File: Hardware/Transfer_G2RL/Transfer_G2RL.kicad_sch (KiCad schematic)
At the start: 20 parts, among them J1 Screw_Terminal_01x02, J5 SO-239, J6 SO-239, J7 SO-239, J8 SO-239, K2 G2RL-1-E, K3 G2RL-1-E

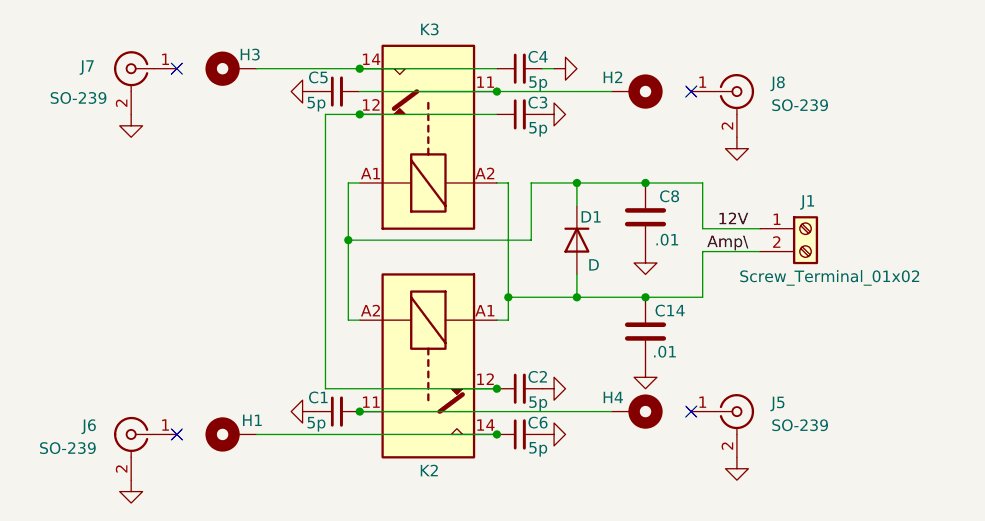
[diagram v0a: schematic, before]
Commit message: replacing through holes with surface pads for RF to coax center pin wires
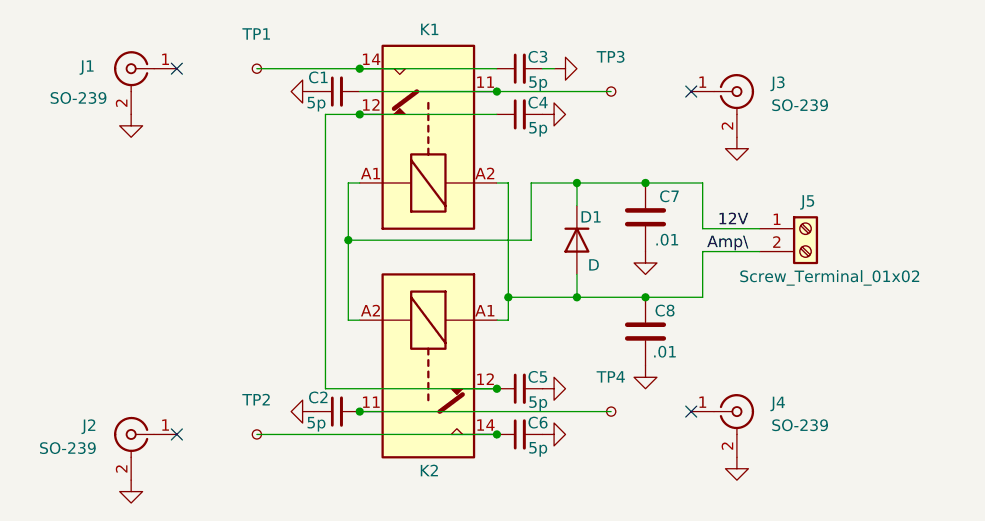
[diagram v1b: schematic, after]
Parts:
- removed H1, H2, H3, H4: MountingHole_Pad, TestPoint:TestPoint_Plated_Hole_D2.0mm, symbol Mechanical:MountingHole_Pad
- added TP1, TP2, TP3, TP4: ~, TestPoint:TestPoint_Pad_3.0x3.0mm, symbol Connector:TestPoint_Small
- renumbered C5 to C1, C1 to C2, C4 to C3, C3 to C4, C2 to C5, C8 to C7, C14 to C8, J7 to J1, J6 to J2, J8 to J3, J5 to J4, J1 to J5, K3 to K1
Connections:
- net at C1.2, K1.11: now also TP3.1
- net at C2.2, K2.11: now also TP4.1
- net at C3.1, K1.14: now also TP1.1
- net at C6.1, K2.14: now also TP2.1

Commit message: Manually merged git branch V2 into main
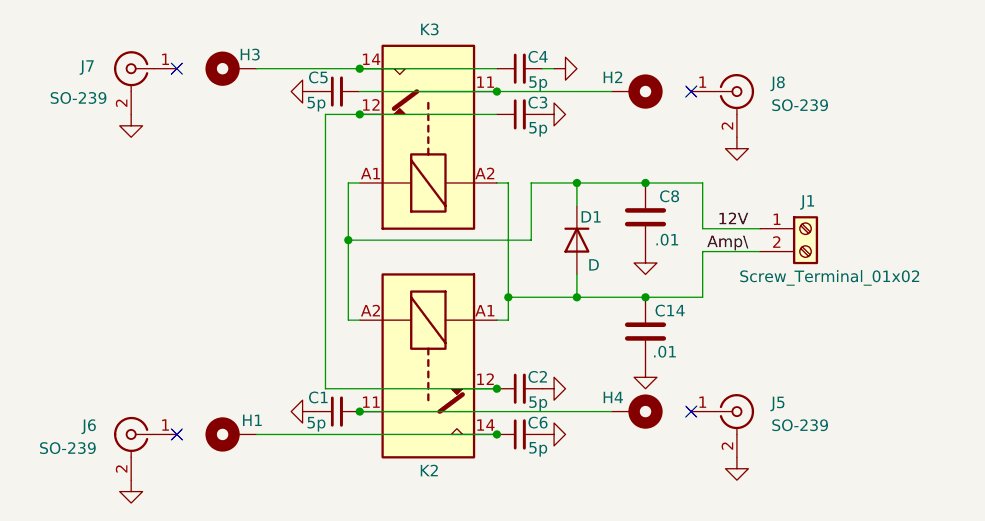
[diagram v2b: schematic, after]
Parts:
- removed TP1, TP2, TP3, TP4: ~, TestPoint:TestPoint_Pad_3.0x3.0mm, symbol Connector:TestPoint_Small
- added H1, H2, H3, H4: MountingHole_Pad, TestPoint:TestPoint_Plated_Hole_D2.0mm, symbol Mechanical:MountingHole_Pad
- renumbered C2 to C1, C8 to C14, C5 to C2, C4 to C3, C3 to C4, C1 to C5, C7 to C8, J5 to J1, J4 to J5, J2 to J6, J1 to J7, J3 to J8, K1 to K3
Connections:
- net at C1.2, K2.11: now also H4.1
- net at C5.2, K3.11: now also H2.1
- net at C4.1, K3.14: now also H3.1
- net at C6.1, K2.14: now also H1.1
